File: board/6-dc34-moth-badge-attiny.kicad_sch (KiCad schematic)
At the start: 13 parts, among them SW3 Mode SW, SW4 ATtiny battery power, U2 ATtiny814-SS

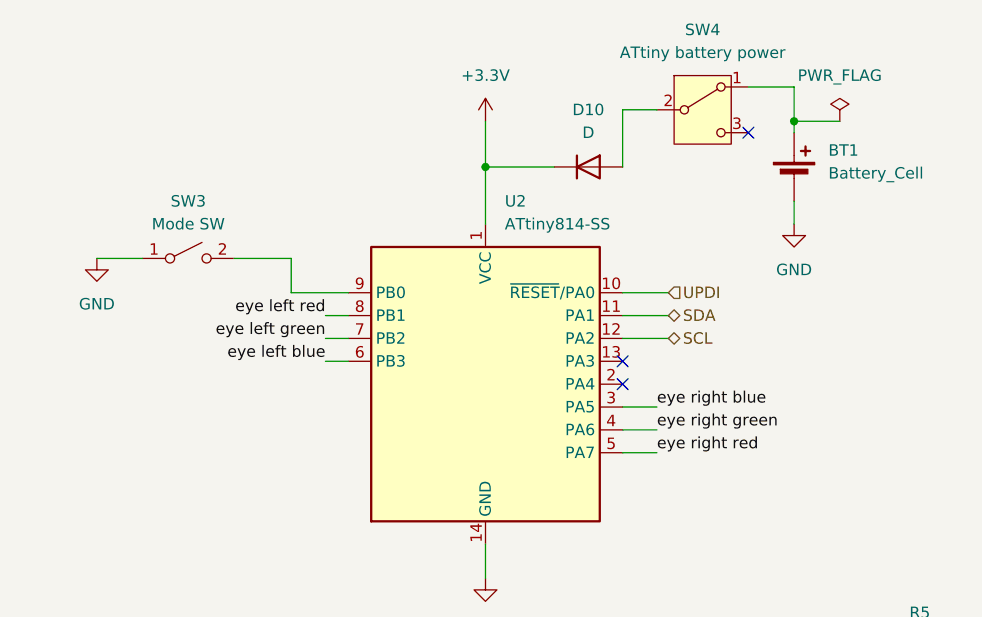
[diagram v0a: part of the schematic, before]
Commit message: board v0.1
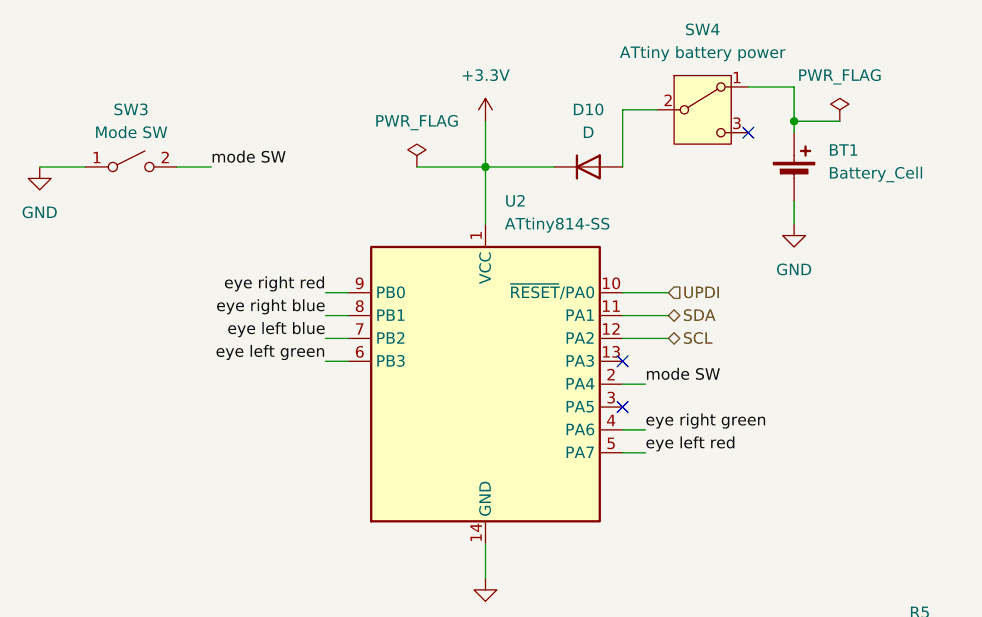
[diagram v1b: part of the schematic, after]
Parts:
- BT1: footprint (none) -> BAT-HLD-001:BATHLD001
- D10: footprint (none) -> Diode_SMD:D_1206_3216Metric_Pad1.42x1.75mm_HandSolder
- D8, D9: footprint (none) -> LED_Osram:KRTBAILMS1A2872
- R10, R5, R6, R7, R8, R9: footprint (none) -> Resistor_SMD:R_1206_3216Metric_Pad1.30x1.75mm_HandSolder
- SW3: footprint (none) -> PHAP3344CR:PHAP3344CR
- SW4: footprint (none) -> SLW-88229-2-SMT-TR:SLW882292SMTTR
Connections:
- net eye left blue: now also U2.7 (PB2); no longer U2.6 (PB3)
- net eye left green: now also U2.6 (PB3); no longer U2.7 (PB2)
- net eye left red: now also U2.5 (PA7); no longer U2.8 (PB1)
- net eye right blue: now also U2.8 (PB1); no longer U2.3 (PA5)
- net eye right red: now also U2.9 (PB0); no longer U2.5 (PA7)
- net mode SW: now reaches U2.2 (PA4)
- net mode SW: now also SW3.2 (B)
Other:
- moved on the sheet: SW3
